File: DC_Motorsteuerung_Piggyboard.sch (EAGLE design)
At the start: 16 parts

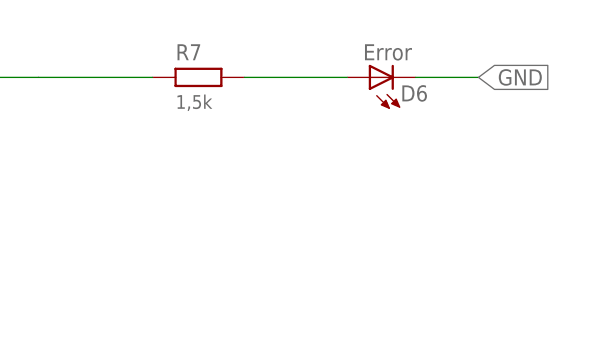
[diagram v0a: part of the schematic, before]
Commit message: Piggiboard updated
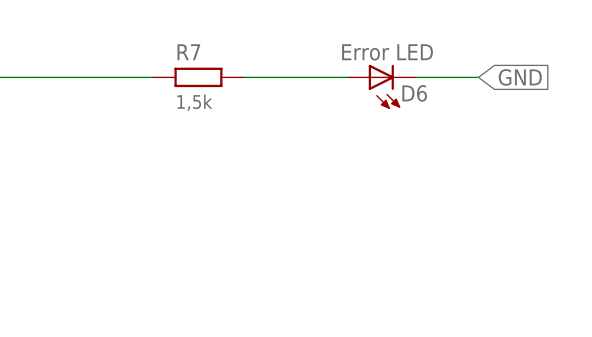
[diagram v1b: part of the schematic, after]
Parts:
- D6: value Error -> Error LED
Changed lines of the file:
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@@
 <part name="SV2" library="con-lstb" deviceset="MA06-2" device=""/>
 <part name="R7" library="Resistor" deviceset="R_0,4W" device="" value="1,5k"/>
-<part name="D6" library="Test" deviceset="LED3MM" device="" value="Error"/>
+<part name="D6" library="Test" deviceset="LED3MM" device="" value="Error LED"/>
 </parts>
 <sheets>
@@
 <instance part="D6" gate="G$1" x="259.715" y="173.99" smashed="yes" rot="R90">
 <attribute name="NAME" x="266.192" y="173.101" size="1.778" layer="95" rot="R180"/>
-<attribute name="VALUE" x="258.953" y="175.895" size="1.778" layer="96"/>
+<attribute name="VALUE" x="256.413" y="175.895" size="1.778" layer="96"/>
 </instance>
 </instances>

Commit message: Piggiboard updated
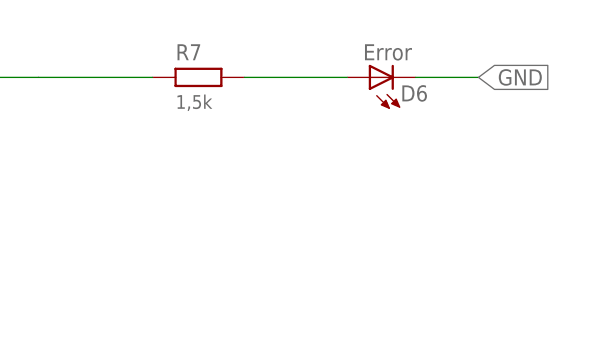
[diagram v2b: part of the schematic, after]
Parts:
- D6: value Error LED -> Error
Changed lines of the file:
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@@
 <part name="SV2" library="con-lstb" deviceset="MA06-2" device=""/>
 <part name="R7" library="Resistor" deviceset="R_0,4W" device="" value="1,5k"/>
-<part name="D6" library="Test" deviceset="LED3MM" device="" value="Error LED"/>
+<part name="D6" library="Test" deviceset="LED3MM" device="" value="Error"/>
 </parts>
 <sheets>
@@
 <instance part="D6" gate="G$1" x="259.715" y="173.99" smashed="yes" rot="R90">
 <attribute name="NAME" x="266.192" y="173.101" size="1.778" layer="95" rot="R180"/>
-<attribute name="VALUE" x="256.413" y="175.895" size="1.778" layer="96"/>
+<attribute name="VALUE" x="258.953" y="175.895" size="1.778" layer="96" font="vector"/>
 </instance>
 </instances>
